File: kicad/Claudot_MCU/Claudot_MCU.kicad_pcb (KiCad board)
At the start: 2 copper layers, 19.1 x 33.3 mm, 37 parts, among them J1 TYPE-C-31-M-12, J2 Conn_01x12, U1 RP2040, U2 W25Q16JVUXIQ, U3 AP2112K-3.3, Y1 12MHz

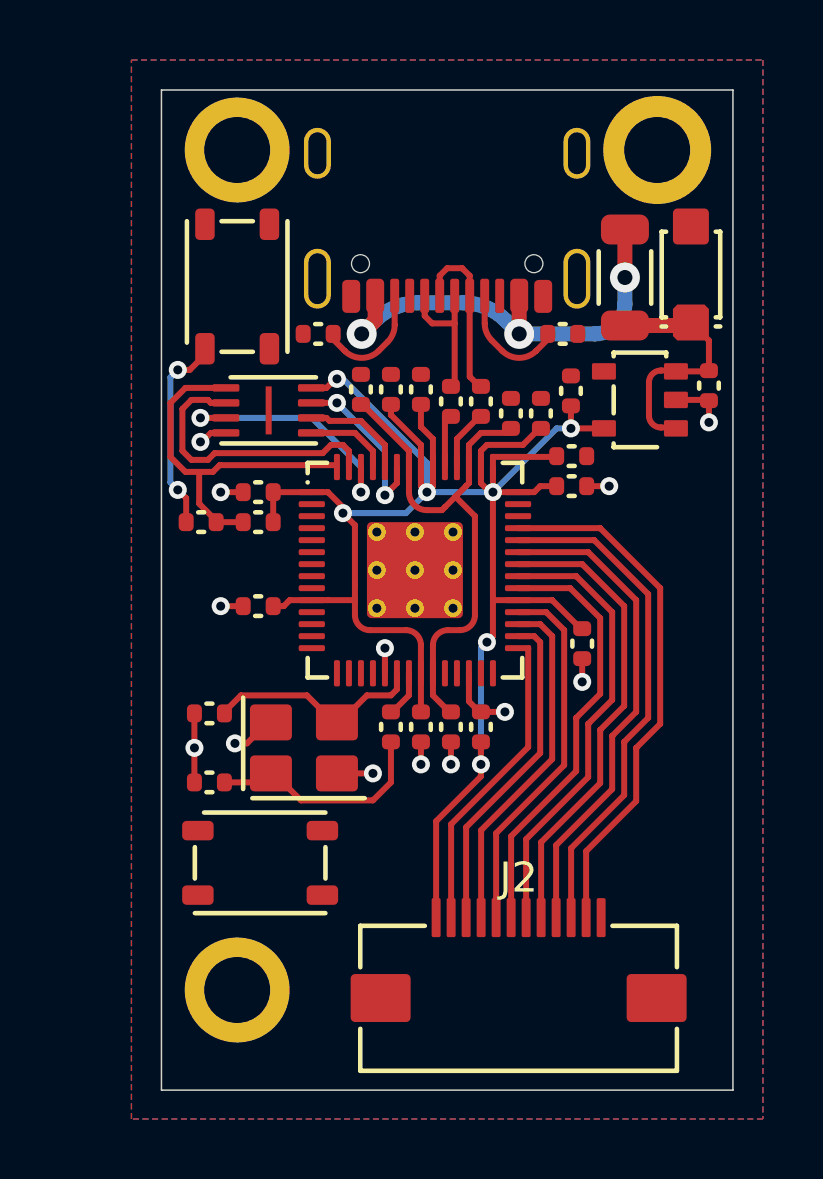
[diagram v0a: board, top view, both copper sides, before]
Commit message: Update schematic and pcb
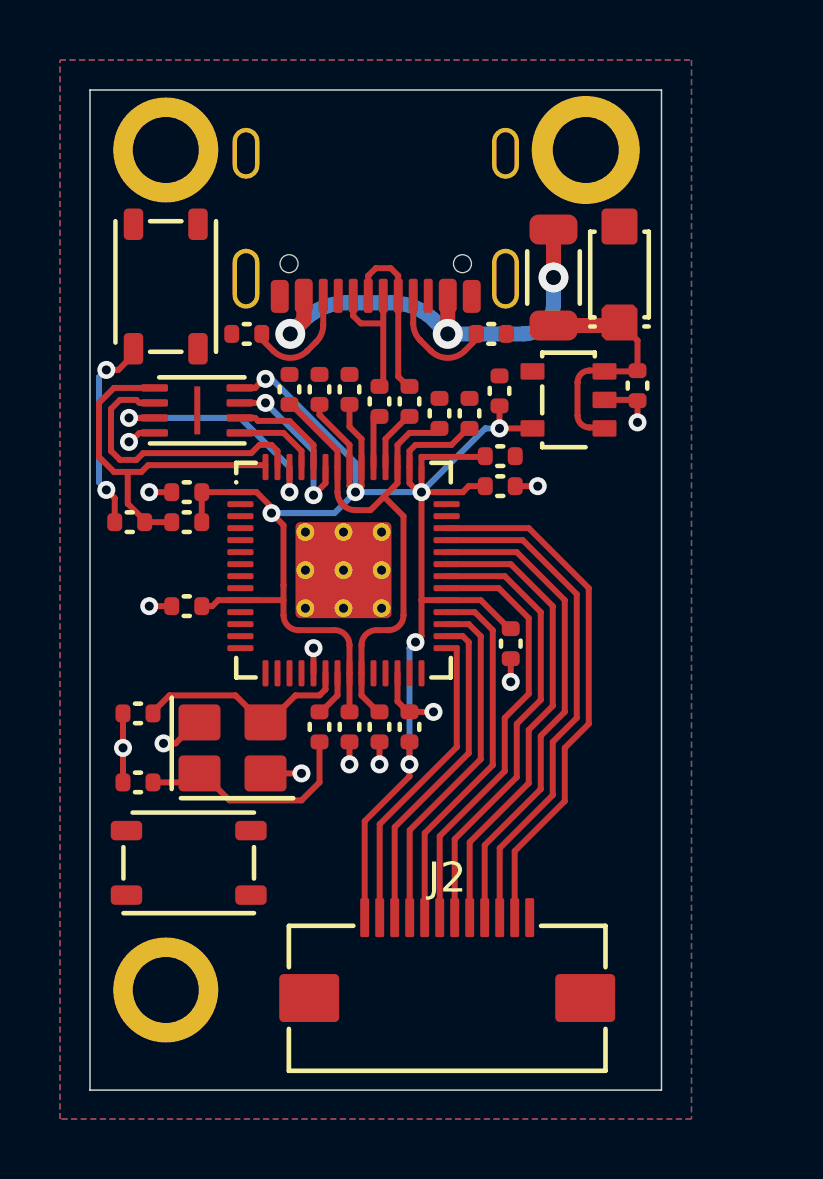
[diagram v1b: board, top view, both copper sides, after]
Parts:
- moved ? 2.38 mm to (147.6, 47.6)
- moved C10 2.38 mm to (142.3, 59.8)
- moved C9 2.38 mm to (142.3, 60.8)
- moved SW_R1 2.38 mm to (131.9, 73.4)
- moved ? 2.38 mm to (131.1, 77.6)
- moved ? 2.38 mm to (131.1, 49.6)
- moved C1 2.38 mm to (130.2, 68.4)
- moved C11 2.38 mm to (137.2, 57.6)
- moved C12 2.38 mm to (136.2, 57.6)
- moved C13 2.38 mm to (138.2, 68.9)
- moved C14 2.38 mm to (135.2, 57.6)
- moved C15 2.38 mm to (146.8, 57.5)
- moved C16 2.38 mm to (142.2, 57.7)
- moved C2 2.38 mm to (130.2, 70.7)
- moved C3 2.38 mm to (141.2, 58.4)
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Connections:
- net D+ renamed DP
- net D- renamed DM
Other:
- board size 19.1 x 33.3 mm -> 19 x 33.3 mm

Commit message: Update MCU pcb
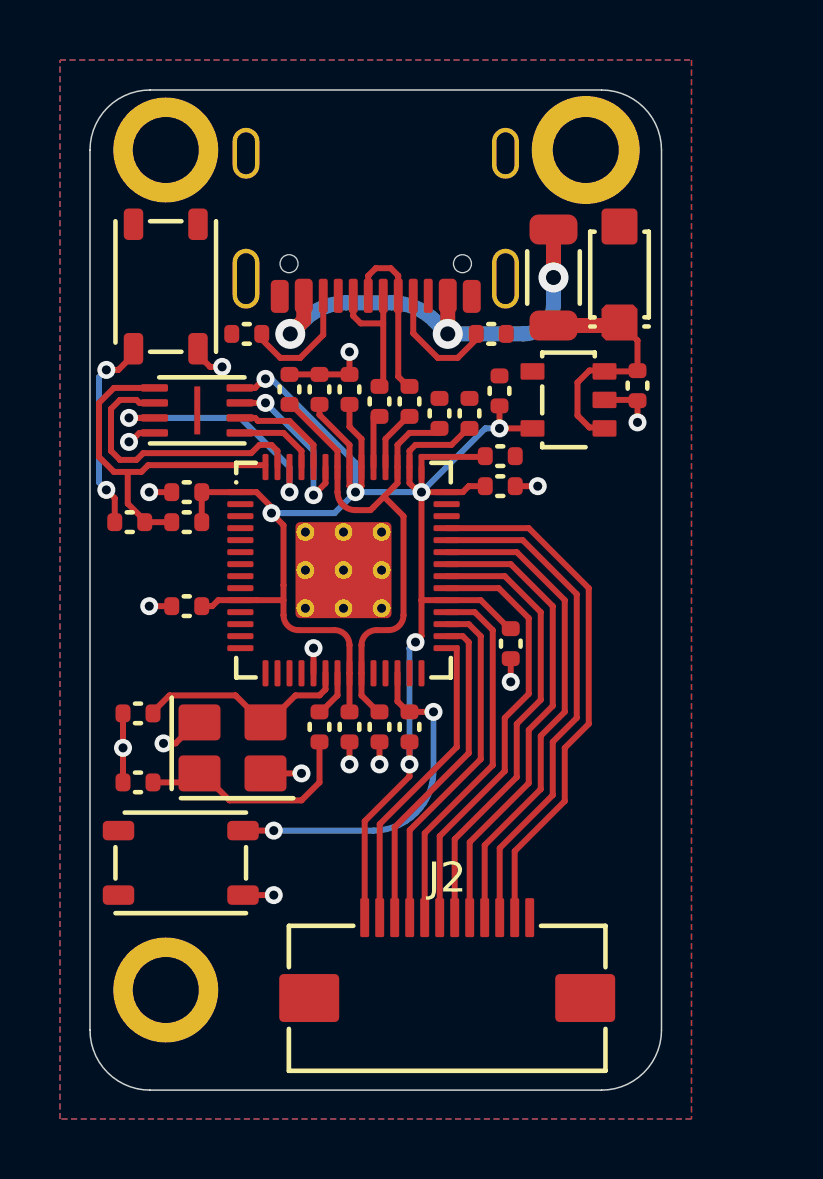
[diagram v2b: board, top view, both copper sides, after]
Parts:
- moved SW1 0.27 mm to (131.6, 73.4)
- renumbered SW_R1 to SW1, SW_B1 to SW2
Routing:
- net ~{RESET}: vias 1 -> 2
- net GND: vias 12 -> 15
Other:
- outline, holes or cut-outs redrawn
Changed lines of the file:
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@@
 	(footprint "Library:SKRP_Switch"
 		(layer "F.Cu")
-		(at 131.877886 73.386921)
+		(at 131.6125 73.386921)
 		(tags "ALPSALPINE, SKRPABE010, C115360")
-		(property "Reference" "SW_R1"
+		(property "Reference" "SW1"
 			(at 0 -2.436 0)
 			(unlocked yes)
@@
 		(at 131.1125 54.175 90)
 		(tags "ALPSALPINE, SKRPABE010, C115360")
-		(property "Reference" "SW_B1"
+		(property "Reference" "SW2"
 			(at 0 -2.436 90)
 			(unlocked yes)
@@
 	(gr_line
 		(start 134.312499 55.936369)
-		(end 134.696815 56.320685)
+		(end 134.931129 56.554999)
 		(stroke
 			(width 0.2)
@@
 		(net 57)
 	)
-	(gr_arc
-		(start 136.3625 55.454999)
-		(mid 136.301604 55.761146)
-		(end 136.128185 56.020685)
+	(gr_line
+		(start 129.2875 59.655)
+		(end 129.5875 59.955)
 		(stroke
 			(width 0.2)
-			(type default)
+			(type solid)
 		)
 		(layer "F.Cu")
-		(net 45)
+		(net 32)
 	)
-	(gr_arc
-		(start 139.596815 55.970685)
-		(mid 139.423397 55.711146)
-		(end 139.3625 55.404999)
+	(gr_line
+		(start 144.8375 57.375)
+		(end 145.2375 56.975)
 		(stroke
 			(width 0.2)
@@
 		)
 		(layer "F.Cu")
-		(net 44)
+		(net 28)
 	)
 	(gr_line
-		(start 129.2875 59.655)
-		(end 129.5875 59.955)
+		(start 132.9925 56.855)
+		(end 132.5925 56.855)
 		(stroke
 			(width 0.2)
@@
 		)
 		(layer "F.Cu")
-		(net 32)
+		(net 9)
 	)
 	(gr_line
@@
 	)
 	(gr_line
-		(start 136.128185 56.020685)
-		(end 135.828185 56.320685)
+		(start 135.593871 56.554999)
+		(end 136.3625 55.78637)
 		(stroke
 			(width 0.2)
@@
 	)
 	(gr_line
+		(start 132.5925 56.855)
+		(end 132.1875 56.45)
+		(stroke
+			(width 0.2)
+			(type solid)
+		)
+		(layer "F.Cu")
+		(net 9)
+	)
+	(gr_line
 		(start 137.8625 53.815)
 		(end 138.1125 53.565)
@@
 	(gr_line
 		(start 136.3625 54.485)
-		(end 136.3625 55.454999)
+		(end 136.3625 55.78637)
 		(stroke
 			(width 0.2)
@@
 	)
 	(gr_line
+		(start 137.2375 57.105)
+		(end 135.2375 57.105)
+		(stroke
+			(width 0.2)
+			(type solid)
+		)
+		(layer "F.Cu")
+		(net 9)
+	)
+	(gr_line
 		(start 134.6375 59.455)
 		(end 134.8375 59.655)
@@
 		(net 22)
 	)
-	(gr_arc
-		(start 145.2375 58.875)
-		(mid 144.954657 58.757843)
-		(end 144.8375 58.475)
-		(stroke
-			(width 0.2)
-			(type default)
-		)
-		(layer "F.Cu")
-		(net 28)
-	)
 	(gr_line
 		(start 146.8375 55.975)
@@
 	)
 	(gr_line
-		(start 139.596815 55.970685)
-		(end 139.946816 56.320685)
+		(start 140.181131 56.554999)
+		(end 139.3625 55.736371)
 		(stroke
 			(width 0.2)
@@
 	)
 	(gr_line
+		(start 140.181131 56.554999)
+		(end 140.84387 56.554999)
+		(stroke
+			(width 0.2)
+			(type default)
+		)
+		(layer "F.Cu")
+		(net 44)
+	)
+	(gr_line
 		(start 132.8625 64.63)
 		(end 133.6 64.63)
@@
 	)
 	(gr_line
+		(start 133.6875 74.461921)
+		(end 134.7125 74.461921)
+		(stroke
+			(width 0.2)
+			(type solid)
+		)
+		(layer "F.Cu")
+		(net 9)
+	)
+	(gr_line
 		(start 129.3875 57.555)
 		(end 130.6375 57.555)
@@
 	)
 	(gr_line
+		(start 137.2375 57.105)
+		(end 137.2375 56.355)
+		(stroke
+			(width 0.2)
+			(type solid)
+		)
+		(layer "F.Cu")
+		(net 9)
+	)
+	(gr_line
 		(start 138.8625 54.485)
 		(end 138.8625 53.815)
@@
 		(net 41)
 	)
-	(gr_arc
-		(start 135.828185 56.320685)
-		(mid 135.2625 56.554999)
-		(end 134.696815 56.320685)
-		(stroke
-			(width 0.2)
-			(type default)
-		)
-		(layer "F.Cu")
-		(net 45)
-	)
 	(gr_line
 		(start 132.3375 70.405)
@@
 		(net 9)
 	)
-	(gr_arc
-		(start 144.8375 57.375)
-		(mid 144.954657 57.092157)
-		(end 145.2375 56.975)
+	(gr_line
+		(start 134.931129 56.554999)
+		(end 135.593871 56.554999)
 		(stroke
 			(width 0.2)
@@
 		)
 		(layer "F.Cu")
-		(net 28)
+		(net 45)
 	)
 	(gr_line
@@
 		(net 9)
 	)
-	(gr_arc
-		(start 141.078185 56.320685)
-		(mid 140.5125 56.554999)
-		(end 139.946815 56.320685)
-		(stroke
-			(width 0.2)
-			(type default)
-		)
-		(layer "F.Cu")
-		(net 44)
-	)
 	(gr_line
 		(start 144.8375 58.475)
@@
 	)
 	(gr_line
+		(start 133.6875 72.311921)
+		(end 134.7125 72.311921)
+		(stroke
+			(width 0.2)
+			(type solid)
+		)
+		(layer "F.Cu")
+		(net 41)
+	)
+	(gr_line
 		(start 134.6375 61.53)
 		(end 134.6375 61.73)
@@
 	(gr_line
 		(start 139.3625 54.485)
-		(end 139.3625 55.404999)
+		(end 139.3625 55.736371)
 		(stroke
 			(width 0.2)
@@
 	)
 	(gr_line
+		(start 145.2375 58.875)
+		(end 144.8375 58.475)
+		(stroke
+			(width 0.2)
+			(type default)
+		)
+		(layer "F.Cu")
+		(net 28)
+	)
+	(gr_line
 		(start 137.6375 60.83)
 		(end 137.6375 60.1925)
@@
 	(gr_line
 		(start 141.4625 55.936369)
-		(end 141.078184 56.320685)
+		(end 140.84387 56.554999)
 		(stroke
 			(width 0.2)
@@
 		(net 43)
 	)
+	(gr_arc
+		(start 140.0375 70.311921)
+		(mid 139.451714 71.726135)
+		(end 138.0375 72.311921)
+		(stroke
+			(width 0.2)
+			(type default)
+		)
+		(layer "B.Cu")
+		(net 41)
+	)
 	(gr_line
 		(start 141.7625 58.905)
@@
 	)
 	(gr_line
+		(start 134.7125 72.311921)
+		(end 138.0375 72.311921)
+		(stroke
+			(width 0.2)
+			(type solid)
+		)
+		(layer "B.Cu")
+		(net 41)
+	)
+	(gr_line
 		(start 139.6375 61.03)
 		(end 137.4375 61.03)
@@
 	)
 	(gr_line
+		(start 140.0375 68.355)
+		(end 140.0375 70.311921)
+		(stroke
+			(width 0.2)
+			(type solid)
+		)
+		(layer "B.Cu")
+		(net 41)
+	)
+	(gr_line
 		(start 138.6483 54.719213)
 		(end 137.126714 54.719213)
@@
 		(layer "Cmts.User")
 	)
-	(gr_rect
-		(start 128.5875 47.625)
-		(end 147.6375 80.9625)
+	(gr_arc
+		(start 147.6375 78.9625)
+		(mid 147.051714 80.376714)
+		(end 145.6375 80.9625)
 		(stroke
 			(width 0.05)
-			(type solid)
+			(type default)
+		)
+		(layer "Edge.Cuts")
+	)
+	(gr_line
+		(start 128.5875 78.9625)
+		(end 128.5875 49.625)
+		(stroke
+			(width 0.05)
+			(type default)
+		)
+		(layer "Edge.Cuts")
+	)
+	(gr_line
+		(start 145.6375 80.9625)
+		(end 130.5875 80.9625)
+		(stroke
+			(width 0.05)
+			(type default)
+		)
+		(layer "Edge.Cuts")
+	)
+	(gr_arc
+		(start 128.5875 49.625)
+		(mid 129.173286 48.210786)
+		(end 130.5875 47.625)
+		(stroke
+			(width 0.05)
+			(type default)
+		)
+		(layer "Edge.Cuts")
+	)
+	(gr_arc
+		(start 145.6375 47.625)
+		(mid 147.051714 48.210786)
+		(end 147.6375 49.625)
+		(stroke
+			(width 0.05)
+			(type default)
+		)
+		(layer "Edge.Cuts")
+	)
+	(gr_line
+		(start 147.6375 49.625)
+		(end 147.6375 78.9625)
+		(stroke
+			(width 0.05)
+			(type default)
+		)
+		(layer "Edge.Cuts")
+	)
+	(gr_arc
+		(start 130.5875 80.9625)
+		(mid 129.173286 80.376714)
+		(end 128.5875 78.9625)
+		(stroke
+			(width 0.05)
+			(type default)
+		)
+		(layer "Edge.Cuts")
+	)
+	(gr_line
+		(start 130.5875 47.625)
+		(end 145.6375 47.625)
+		(stroke
+			(width 0.05)
+			(type default)
 		)
-		(fill no)
 		(layer "Edge.Cuts")
 	)
@@
 	)
 	(via
+		(at 137.2375 56.355)
+		(size 0.6)
+		(drill 0.3)
+		(layers "F.Cu" "B.Cu")
+		(remove_unused_layers yes)
+		(keep_end_layers yes)
+		(zone_layer_connections)
+		(net 9)
+	)
+	(via
+		(at 134.7125 74.461921)
+		(size 0.6)
+		(drill 0.3)
+		(layers "F.Cu" "B.Cu")
+		(remove_unused_layers yes)
+		(keep_end_layers yes)
+		(zone_layer_connections)
+		(net 9)
+	)
+	(via
 		(at 136.0375 66.23)
 		(size 0.6)
@@
 	)
 	(via
+		(at 132.9925 56.855)
+		(size 0.6)
+		(drill 0.3)
+		(layers "F.Cu" "B.Cu")
+		(remove_unused_layers yes)
+		(keep_end_layers yes)
+		(zone_layer_connections)
+		(net 9)
+	)
+	(via
 		(at 130.5625 61.03)
 		(size 0.6)
@@
 		(size 0.6)
 		(drill 0.3)
+		(layers "F.Cu" "B.Cu")
+		(remove_unused_layers yes)
+		(keep_end_layers yes)
+		(zone_layer_connections)
+		(net 41)
+	)
+	(via
+		(at 134.7125 72.311921)
+		(size 0.6)
+		(drill 0.3)
